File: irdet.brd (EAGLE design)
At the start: 50.8 x 47.9 mm, 66 parts, among them IC1 MEGA8-AI, IC2 78L05F, J1 PSH02-04WG, J2 PSH02-04WG, J3 PSH02-04WG, J4 PSH02-04WG, J5 22-05-7098-09, T1 S9013, T2 S9012, T3 S9013, T4 S9012, T5 S9013, T6 S9012, T7 S9013, T8 S9012, X1 ARK500/2

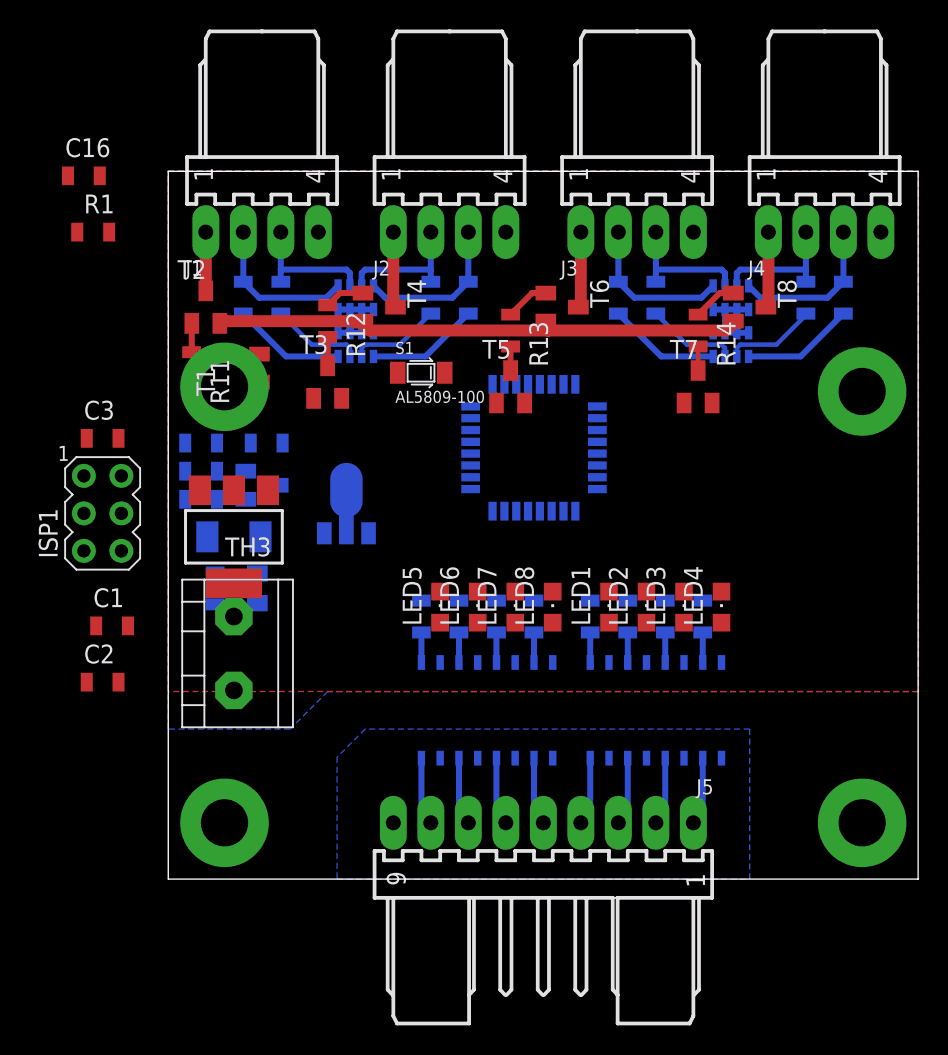
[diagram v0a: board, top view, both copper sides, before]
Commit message: Add rest of PCB.
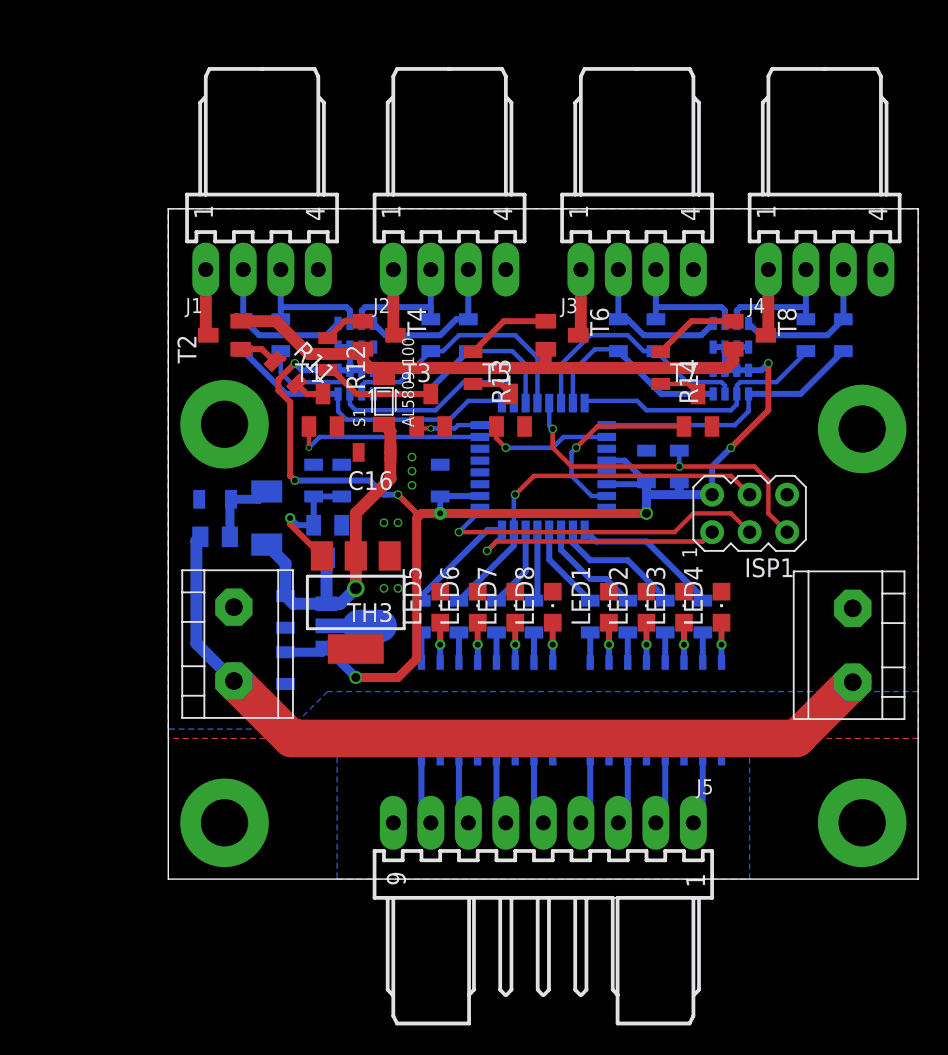
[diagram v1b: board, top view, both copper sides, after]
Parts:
- removed C3: 100n, rcl:C0805
- added X2: ARK500/2, con-malina:ARK500/2
- moved ISP1 43.8 mm to (39.4, 24.8), turned to 90 degrees
- moved R1 42.7 mm to (34.6, 27.9), flipped to the bottom, turned to 270 degrees
- moved C2 39.6 mm to (32.4, 27.9), flipped to the bottom, turned to 270 degrees
- moved C16 27.2 mm to (14.0, 28.9), turned to 180 degrees
- moved C1 24.3 mm to (18.4, 27.0), flipped to the bottom, turned to 270 degrees
- moved C8 15.3 mm to (7.94, 14.3), turned to 270 degrees
- moved C7 12.8 mm to (7.94, 18.1), turned to 270 degrees
- moved R2 9.55 mm to (11.7, 27.0), turned to 270 degrees
- moved TH3 9.38 mm to (12.7, 18.7)
- moved IC2 8.28 mm to (12.7, 17.1), turned to 90 degrees
- moved C13 7.73 mm to (9.84, 27.0), turned to 90 degrees
- moved T3 7.24 mm to (17.8, 31.8)
- moved R11 6.36 mm to (7.94, 34.3), turned to 315 degrees
- moved T1 6.11 mm to (10.5, 31.8), turned to 0 degrees
- moved C12 6.03 mm to (3.17, 25.7), turned to 0 degrees
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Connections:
- removed net MISO: IC1.16, ISP1.1
- removed net MOSI/IN7: C14.1, IC1.15, ISP1.4, RN4.2
- removed net N$34: F1.1, X1.1
- removed net OUT1: IC1.30, R3.1
- removed net OUT2: IC1.31, R4.1
- new net +12VIN: F1.1, X1.2, X2.1
- new net IN7: C14.1, IC1.32, RN4.2
- new net MISO/OUT1: IC1.16, ISP1.1, R7.1
- new net MOSI/OUT2: IC1.15, ISP1.4, R8.1
- net +5V: no longer C3.1
- net CPUPOW1-2: now also IC1.23; no longer IC1.12
- net CPUPOW3-4: now also IC1.24; no longer IC1.13
- net CPUPOW5-6: now also IC1.2; no longer IC1.14
- net GND: now also X1.1, X2.2; no longer C3.2, X1.2
- net IN1: now also IC1.25; no longer IC1.23
- net IN2: now also IC1.26; no longer IC1.24
- net IN3: now also IC1.28; no longer IC1.25
- net IN4: now also IC1.27; no longer IC1.26
- net IN5: now also IC1.31; no longer IC1.27
- net IN6: now also IC1.30; no longer IC1.28
- net IN8: now also IC1.1; no longer IC1.8
- net OUT3: now also IC1.14, R9.1; no longer IC1.32, R5.1
- net OUT4: now also IC1.13, R10.1; no longer IC1.1, R6.1
- net OUT5: now also IC1.12, R3.1; no longer IC1.2, R7.1
- net OUT6: now also IC1.11, R4.1; no longer IC1.9, R8.1
- net OUT7: now also R5.1; no longer R9.1
- net OUT8: now also IC1.9, R6.1; no longer IC1.11, R10.1
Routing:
- net +5V: track 12.8 -> 99.1 mm, vias 0 -> 8
- net +12VIN: track 0.00 -> 56.0 mm
- net MOSI/OUT2: track 0.00 -> 25.7 mm, vias 0 -> 1
- net MISO/OUT1: track 0.00 -> 25.2 mm, vias 0 -> 1
- net +12V: track 0.00 -> 24.8 mm, vias 0 -> 1
- net RST: track 0.00 -> 23.7 mm, vias 0 -> 2
- net SCK: track 0.00 -> 23.0 mm, vias 0 -> 1
- net IN7: track 0.00 -> 17.8 mm
- net IN2: track 6.21 -> 20.9 mm
- net CPUPOW1-2: track 0.00 -> 13.3 mm, vias 0 -> 1
- net IN1: track 7.62 -> 20.7 mm
- net CPUPOW7-8: track 0.00 -> 12.9 mm, vias 0 -> 1
- net IN3: track 6.21 -> 17.6 mm
- net IN8: track 7.62 -> 18.8 mm
- net IN6: track 6.21 -> 16.5 mm
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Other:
- board size 50.8 x 47.9 mm -> 50.8 x 45.4 mm
